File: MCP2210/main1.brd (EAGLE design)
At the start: 26 x 18.7 mm, 12 parts, among them J1 USB_A_SMT_MALE, Q1 12MHz

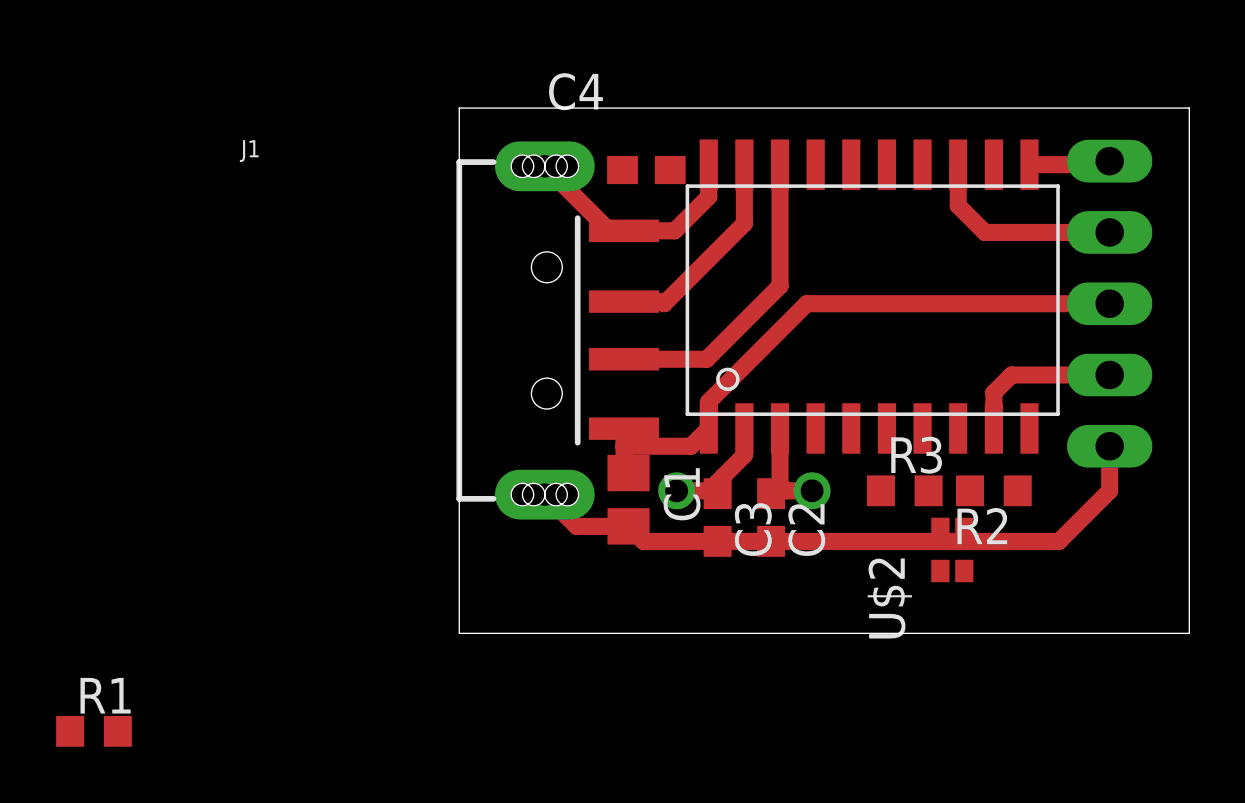
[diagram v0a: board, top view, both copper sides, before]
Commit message: started new layout
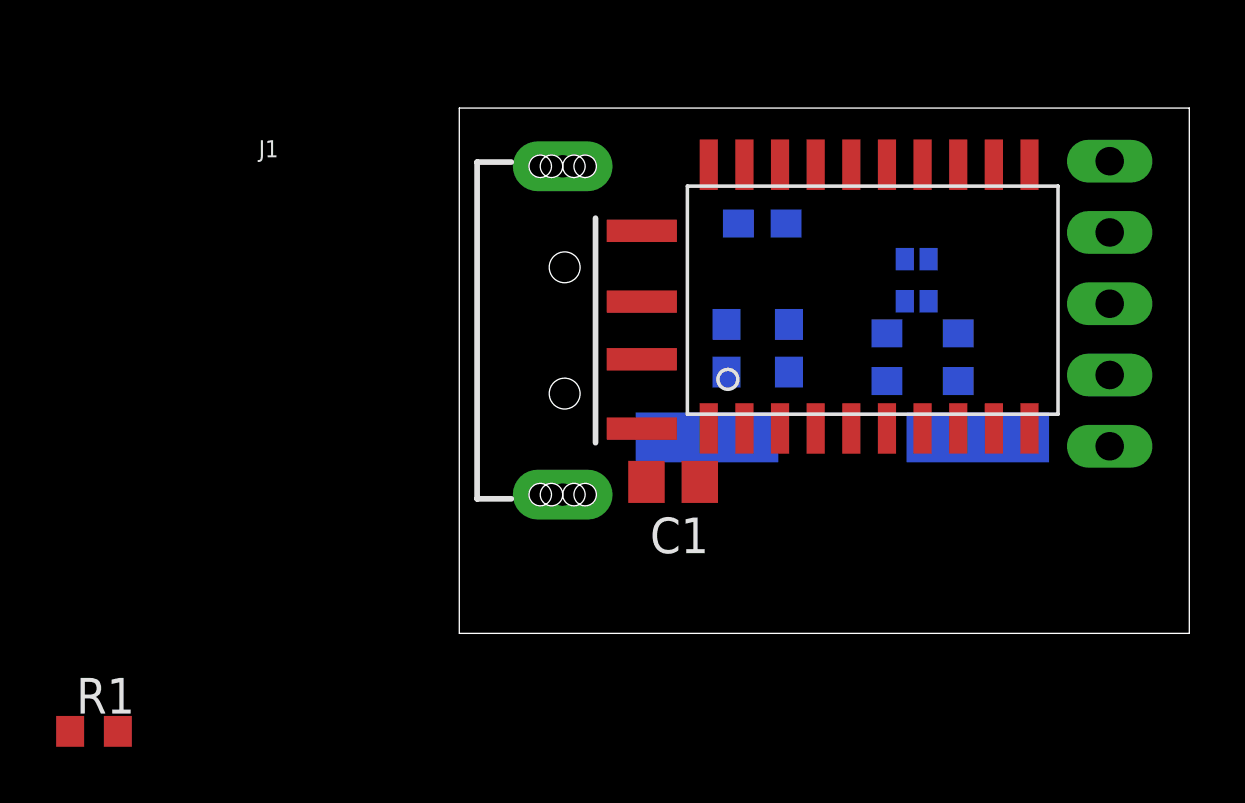
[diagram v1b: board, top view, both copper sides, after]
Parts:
- Q1: device crystal:HC49U-V -> crystal:SM49
- moved U$2 11.2 mm to (15.9, 8.89), flipped to the bottom, turned to 270 degrees
- moved C2 6.07 mm to (11.7, 5.71), flipped to the bottom, turned to 90 degrees
- moved C3 6.04 mm to (9.53, 5.71), flipped to the bottom, turned to 90 degrees
- moved R2 4.93 mm to (17.8, 5.40), flipped to the bottom, turned to 90 degrees
- moved R3 4.80 mm to (15.2, 5.40), flipped to the bottom, turned to 270 degrees
- moved C4 4.55 mm to (10.8, 10.2), flipped to the bottom
- moved Q1 3.98 mm to (13.7, 2.54)
- moved C1 1.71 mm to (7.62, 0.95), turned to 180 degrees
- moved J1 0.63 mm to (-4.45, 6.35)
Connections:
- net N$1 renamed N+
- net N$2 renamed N-
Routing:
- net N$3: track 31.9 -> 0.00 mm
- net N$4: track 21.6 -> 0.00 mm
- net N-: track 11.0 -> 0.00 mm
- net N+: track 7.60 -> 0.00 mm
- net N$14: track 7.25 -> 0.00 mm
- net N$15: track 5.66 -> 0.00 mm
- net N$5: track 3.89 -> 0.00 mm
- net N$6: track 3.69 -> 0.00 mm
- net N$13: track 2.91 -> 0.00 mm

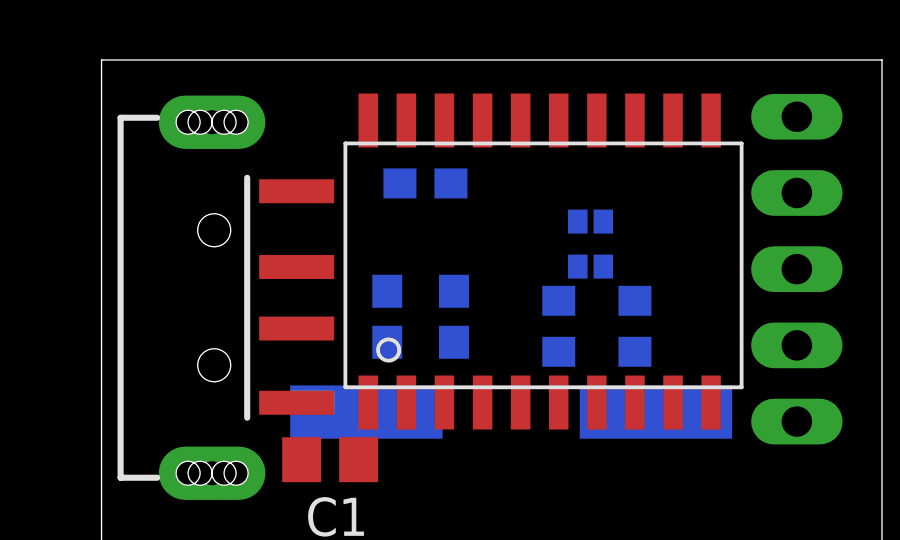
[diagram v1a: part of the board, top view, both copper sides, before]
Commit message: -ma
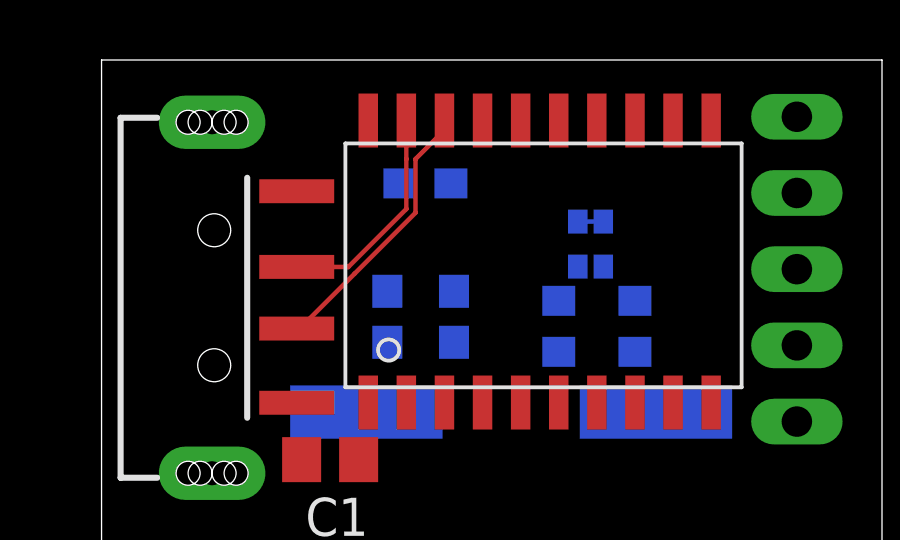
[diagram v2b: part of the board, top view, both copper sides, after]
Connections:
- net N+ renamed N_P
- net N- renamed N_N
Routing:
- net N_N: track 0.00 -> 9.03 mm
- net N_P: track 0.00 -> 7.41 mm
- net N$4: track 0.00 -> 0.85 mm
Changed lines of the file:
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@@
 <setting verticaltext="up"/>
 </settings>
-<grid distance="12.5" unitdist="mil" unit="mil" style="dots" multiple="1" display="yes" altdistance="5" altunitdist="mil" altunit="mil"/>
+<grid distance="2" unitdist="mil" unit="mil" style="dots" multiple="1" display="yes" altdistance="5" altunitdist="mil" altunit="mil"/>
 <layers>
 <layer number="1" name="Top" color="4" fill="1" visible="yes" active="yes"/>
@@
 </elements>
 <signals>
-<signal name="N+">
+<signal name="N_P">
 <contactref element="U$1" pad="19"/>
 <contactref element="J1" pad="D+1"/>
-<wire x1="6.505" y1="7.377" x2="10.16" y2="12.2575" width="0" layer="19" extent="1-1"/>
+<wire x1="6.505" y1="7.377" x2="8.2186" y2="7.377" width="0.1524" layer="1"/>
+<wire x1="8.2186" y1="7.377" x2="8.223434375" y2="7.372165625" width="0.1524" layer="1"/>
+<wire x1="8.223434375" y1="7.372165625" x2="10.16" y2="9.30873125" width="0.1524" layer="1"/>
+<wire x1="10.16" y1="9.30873125" x2="10.16" y2="10.9728" width="0.1524" layer="1"/>
+<wire x1="10.16" y1="12.2575" x2="10.16" y2="10.9728" width="0.1524" layer="1"/>
 </signal>
-<signal name="N-">
+<signal name="N_N">
 <contactref element="U$1" pad="18"/>
 <contactref element="J1" pad="D-1"/>
-<wire x1="6.505" y1="5.323" x2="11.43" y2="12.2575" width="0" layer="19" extent="1-1"/>
+<wire x1="6.505" y1="5.323" x2="6.60533125" y2="5.323" width="0.1524" layer="1"/>
+<wire x1="6.60533125" y1="5.323" x2="8.438965625" y2="7.156634375" width="0.1524" layer="1"/>
+<wire x1="8.438965625" y1="7.156634375" x2="10.4648" y2="9.18246875" width="0.1524" layer="1"/>
+<wire x1="10.4648" y1="9.18246875" x2="10.4648" y2="10.9728" width="0.1524" layer="1"/>
+<wire x1="10.4648" y1="10.9728" x2="11.43" y2="11.938" width="0.1524" layer="1"/>
+<wire x1="11.43" y1="11.938" x2="11.43" y2="12.2575" width="0.1524" layer="1"/>
 </signal>
 <signal name="N$3">
@@
 <contactref element="SV1" pad="3"/>
 <contactref element="R1" pad="2"/>
+<wire x1="15.875" y1="8.89" x2="16.725" y2="8.89" width="0.1524" layer="16"/>
 <wire x1="16.725" y1="8.89" x2="23.1775" y2="7.3025" width="0" layer="19" extent="16-16"/>
-<wire x1="15.875" y1="8.89" x2="16.725" y2="8.89" width="0" layer="19" extent="16-16"/>
 <wire x1="8.89" y1="2.8575" x2="15.875" y2="8.89" width="0" layer="19" extent="1-16"/>
 <wire x1="8.57" y1="0.9525" x2="8.89" y2="2.8575" width="0" layer="19" extent="1-1"/>
